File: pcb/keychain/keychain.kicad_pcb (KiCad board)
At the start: 2 copper layers, 43.2 x 30.5 mm, 11 parts, among them J2 AVR-ISP-6, J3 Vin, U1 ATtiny84A-SS, U3 LM1117MP-3.3

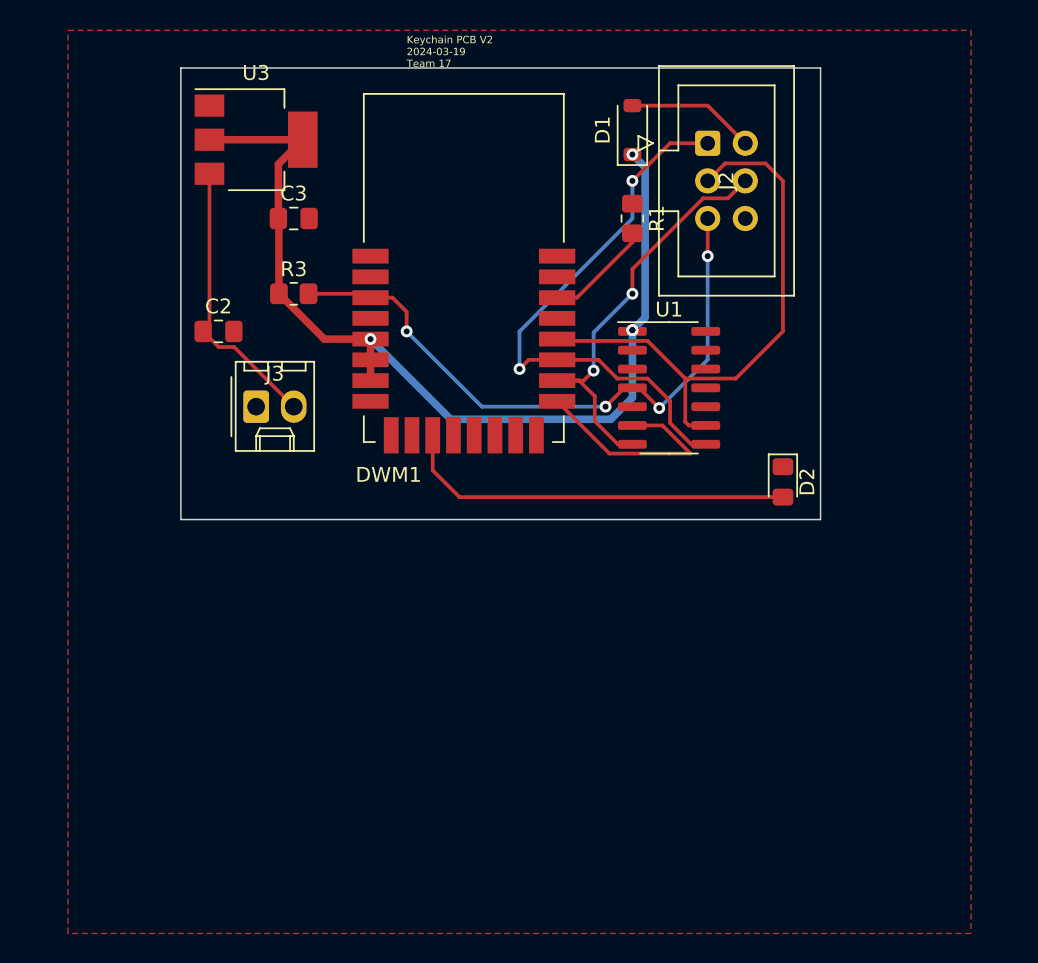
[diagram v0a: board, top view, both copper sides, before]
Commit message: dish pcb updated
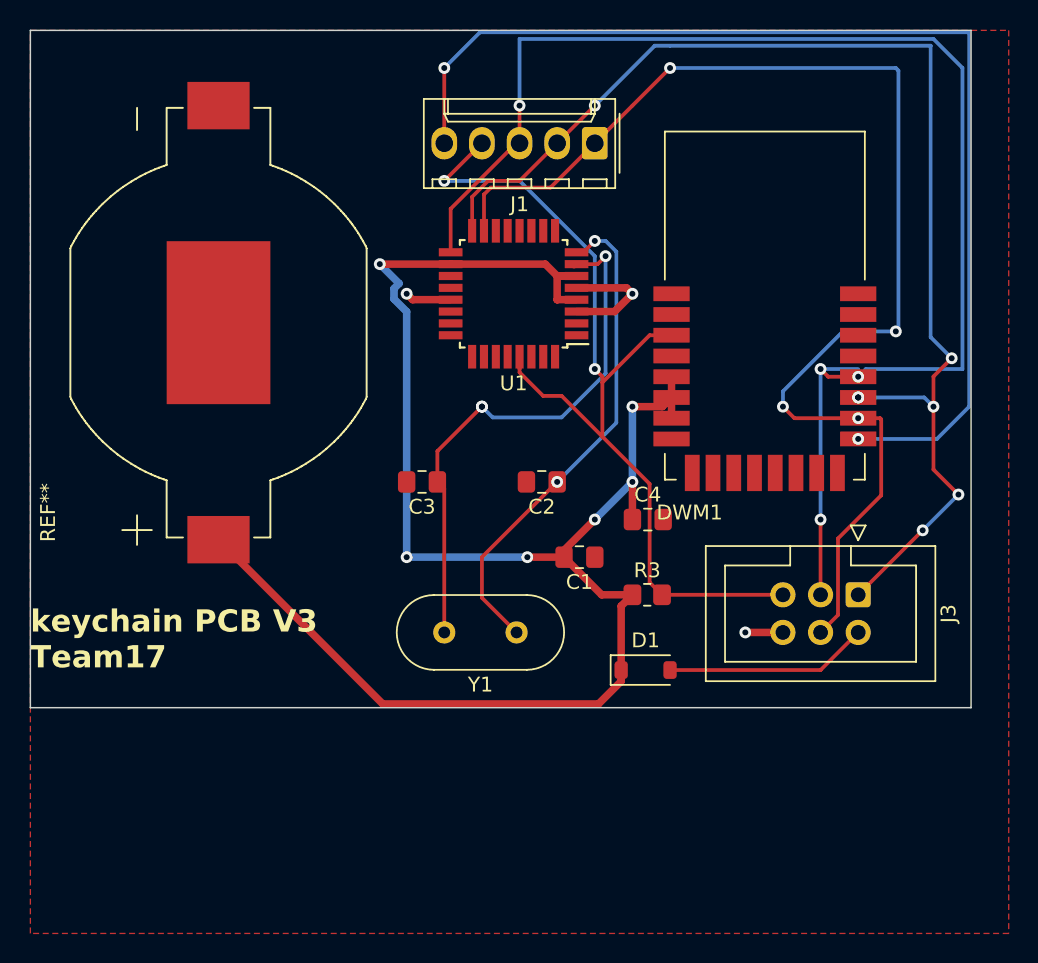
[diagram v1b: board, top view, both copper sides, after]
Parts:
- removed D2: LED, LED_SMD:LED_0805_2012Metric_Pad1.15x1.40mm_HandSolder
- removed J2: AVR-ISP-6, Connector_IDC:IDC-Header_2x03_P2.54mm_Vertical
- removed R1: 100, Resistor_SMD:R_0805_2012Metric_Pad1.20x1.40mm_HandSolder
- removed U3: LM1117MP-3.3, Package_TO_SOT_SMD:SOT-223-3_TabPin2
- added C1: 1uF, Capacitor_SMD:C_0805_2012Metric_Pad1.18x1.45mm_HandSolder, F.Cu at (136.1, 86.4)
- added C4: 10uF, Capacitor_SMD:C_0805_2012Metric_Pad1.18x1.45mm_HandSolder, F.Cu at (140.7, 83.8)
- added J1: Conn_01x05, Connector_Molex:Molex_KK-254_AE-6410-05A_1x05_P2.54mm_Vertical, F.Cu at (137.2, 58.4)
- added REF**: BAT_BU2032SM-HD-G, BU2032SM_HD_G:BAT_BU2032SM-HD-G, F.Cu at (111.8, 70.5)
- added Y1: 16MHz, Crystal:Crystal_HC49-U_Vertical, F.Cu at (131.9, 91.4)
- C2, C3: value 10uF -> 22p
- J3: value Vin -> AVR-ISP-6; footprint Connector_Molex:Molex_KK-254_AE-6410-02A_1x02_P2.54mm_Vertical -> Connector_IDC:IDC-Header_2x03_P2.54mm_Vertical
- U1: value ATtiny84A-SS -> ATmega328-A; footprint Package_SO:SOIC-14_3.9x8.7mm_P1.27mm -> Package_QFP:TQFP-32_7x7mm_P0.8mm
- moved J3 42.6 mm to (154.9, 88.9), turned to -90 degrees
- moved D1 36.5 mm to (140.6, 94.0), turned to 0 degrees
- moved R3 31.3 mm to (140.7, 88.9)
- moved C2 24.1 mm to (133.6, 81.3), turned to 180 degrees
- moved DWM1 20.5 mm to (148.6, 69.4)
- moved C3 19.8 mm to (125.5, 81.3), turned to 180 degrees
- moved U1 12.3 mm to (131.7, 68.6), turned to 180 degrees
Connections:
- C2 pad 1: Net-(J3-Pin_2) -> Net-(U1-XTAL2/PB7)
- C3 pad 1: +3.3V -> Net-(U1-XTAL1/PB6)
- DWM1 pad 11: Net-(D2-A) -> unconnected-(DWM1-GPIO4/EXTPA-Pad11)
- DWM1 pad 22: /interrupt -> unconnected-(DWM1-IRQ/GPIO8-Pad22)
- DWM1 pad 3: /RST -> /RESET
- J3 pad 1: GND -> /MISO
- J3 pad 2: Net-(J3-Pin_2) -> Net-(D1-A)
- R3 pad 2: /RST -> /RESET
- U1 pad 1: +3.3V -> unconnected-(U1-PD3-Pad1)
- U1 pad 14: GND -> unconnected-(U1-PB2-Pad14)
- U1 pad 3: unconnected-(U1-XTAL2/PB1-Pad3) -> GND
- U1 pad 4: /RST -> +3.3V
- U1 pad 5: unconnected-(U1-PB2-Pad5) -> GND
- U1 pad 6: /Csn -> +3.3V
- U1 pad 7: /MOSI -> Net-(U1-XTAL1/PB6)
- U1 pad 8: /MISO -> Net-(U1-XTAL2/PB7)
- U1 pad 9: /SCK -> unconnected-(U1-PD5-Pad9)
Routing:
- net /RESET: track 0.00 -> 64.0 mm, vias 0 -> 2
- net /Csn: track 15.2 -> 75.7 mm, vias 0 -> 2
- net /MOSI: track 28.6 -> 85.1 mm, vias 2 -> 4
- net /SCK: track 39.3 -> 95.3 mm, vias 0 -> 4
- net +3.3V: track 65.4 -> 113.8 mm, vias 4 -> 6
- net /MISO: track 38.0 -> 84.5 mm, vias 2 -> 7
- net /RST: track 42.8 -> 0.00 mm, vias 4 -> 0
- net Net-(U1-XTAL1/PB6): track 0.00 -> 36.9 mm, vias 0 -> 3
- net Net-(U1-XTAL2/PB7): track 0.00 -> 33.7 mm, vias 0 -> 2
- net Net-(D2-A): track 26.8 -> 0.00 mm
- net Net-(J3-Pin_2): track 19.0 -> 0.00 mm
- net GND: track 0.00 -> 13.9 mm, vias 0 -> 3
- net /interrupt: track 7.23 -> 0.00 mm
- net Net-(D1-A): track 8.67 -> 13.8 mm
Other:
- board size 43.2 x 30.5 mm -> 63.5 x 45.7 mm
- board text added: "keychain PCB V3 Team17"
- board text removed: "Keychain PCB V2 2024-03-19 Team 17"
